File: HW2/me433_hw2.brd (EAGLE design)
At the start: 50 x 50 mm, 22 parts

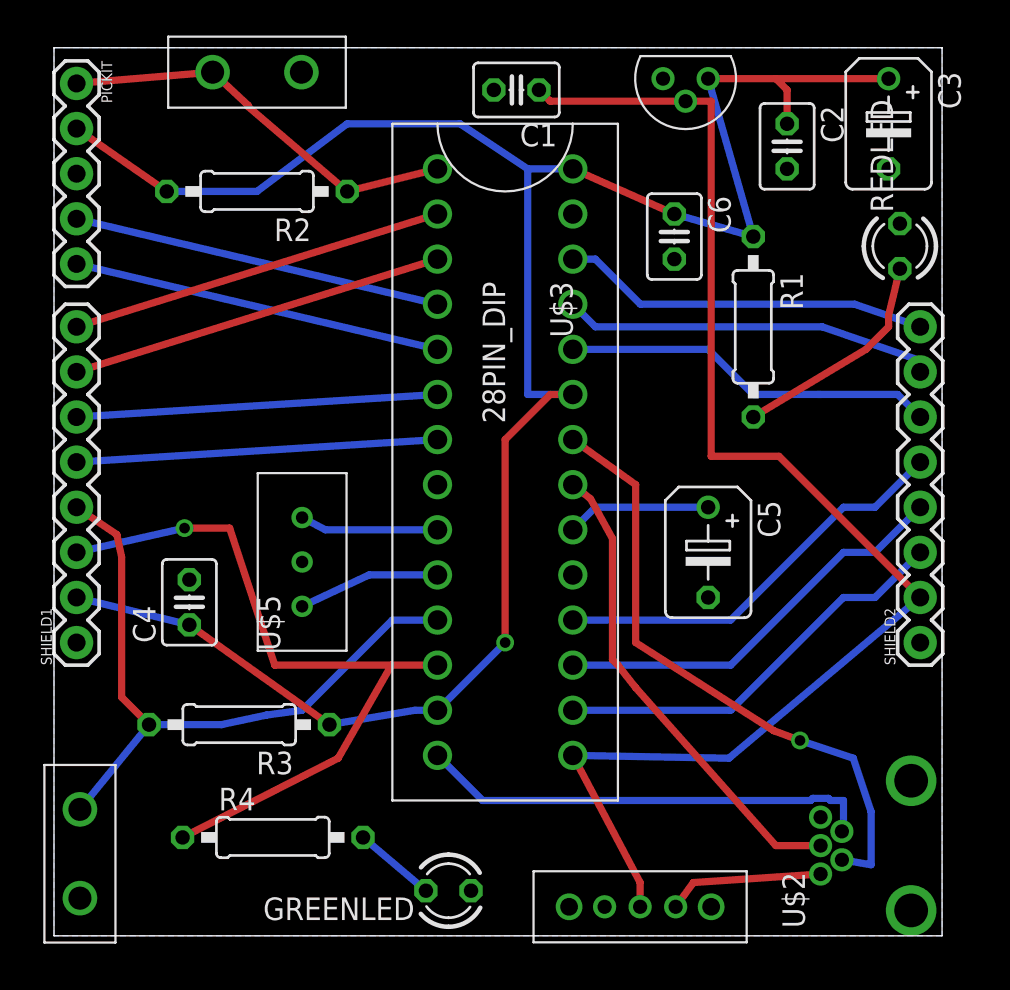
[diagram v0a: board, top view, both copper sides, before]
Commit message: finished pcb and gerber files
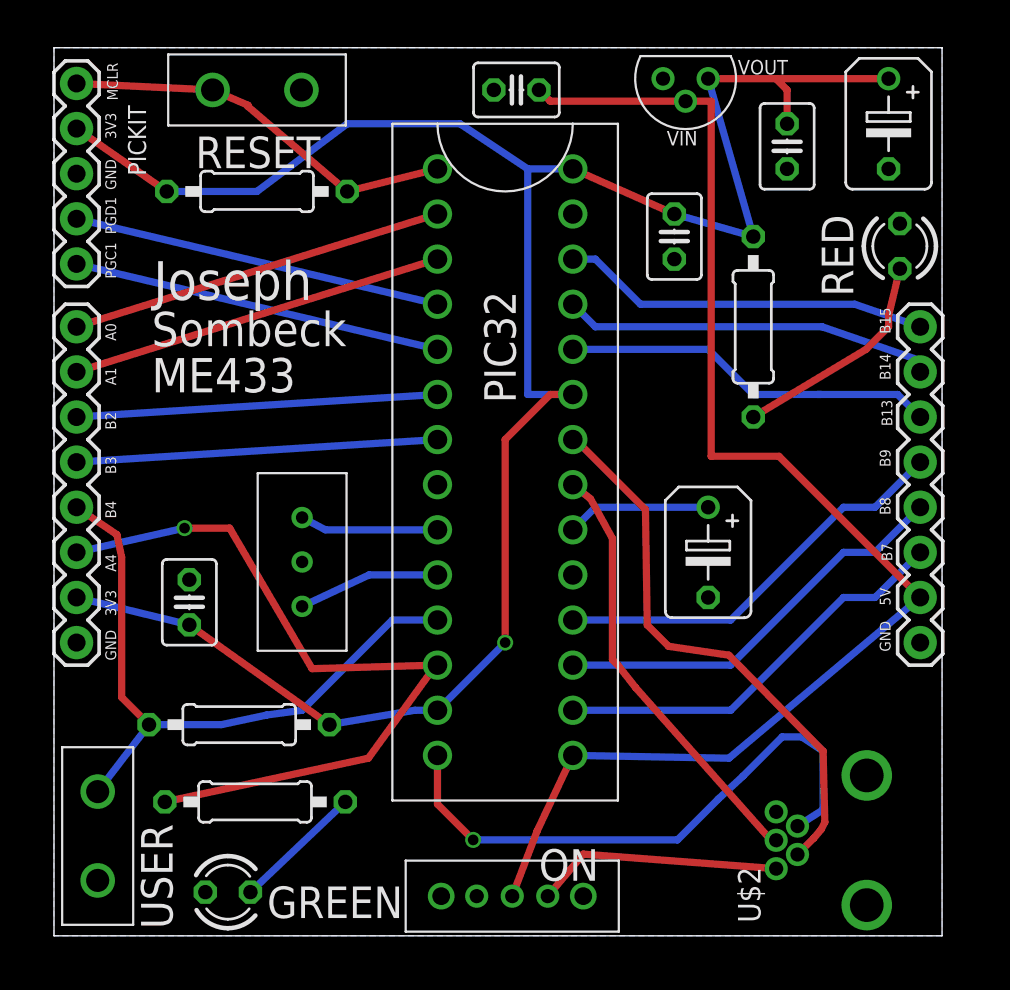
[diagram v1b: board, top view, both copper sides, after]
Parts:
- moved GREENLED 12.4 mm to (9.79, 2.46), turned to 0 degrees
- moved U$4 7.22 mm to (25.8, 2.23)
- moved U$2 2.52 mm to (45.8, 5.38)
- moved R4 2.24 mm to (11.3, 7.54)
- moved USER 1.41 mm to (2.46, 5.62)
- moved RESET 1.00 mm to (11.4, 47.6)
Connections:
- net GND: no longer U$4.RIGHT
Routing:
- net USBID: track 25.8 -> 32.9 mm, vias 0 -> 1
- net SLIDESWITCH: track 8.87 -> 14.0 mm
- net D-: track 35.0 -> 31.3 mm, vias 1 -> 0
- net N$6: track 4.64 -> 7.37 mm
- net D+: track 27.1 -> 24.9 mm
- net B4: track 38.7 -> 37.3 mm
- net A4: track 41.9 -> 43.2 mm
- net +5V: track 77.3 -> 76.5 mm
- net MCLR: track 23.1 -> 22.5 mm
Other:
- board text added: "3V3"
- board text added: "5V"
- board text added: "A0"
- board text added: "A1"
- board text added: "A4"
- board text added: "B13"
- board text added: "B14"
- board text added: "B15"
- board text added: "B2"
- board text added: "B3"
- board text added: "B4"
- board text added: "B7"
- board text added: "B8"
- board text added: "B9"
- board text added: "GND"
- board text added: "GREEN"
- board text added: "Joseph"
- board text added: "MCLR"
- board text added: "ME433"
- board text added: "ON"
- board text added: "PGC1"
- board text added: "PGD1"
- board text added: "PIC32"
- board text added: "RED"
- board text added: "RESET"
- board text added: "Sombeck"
- board text added: "USER"
- board text added: "VIN"
- board text added: "VOUT"
